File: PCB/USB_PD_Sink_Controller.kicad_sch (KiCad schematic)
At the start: 28 parts, among them J1 USB_C_Receptacle_PowerOnly_6P, J2 JST_01x02_Socket, J3 JST_01x05_Socket, U1 STUSB4500QTR, U2 STL6P3LLH6, U3 STL6P3LLH6

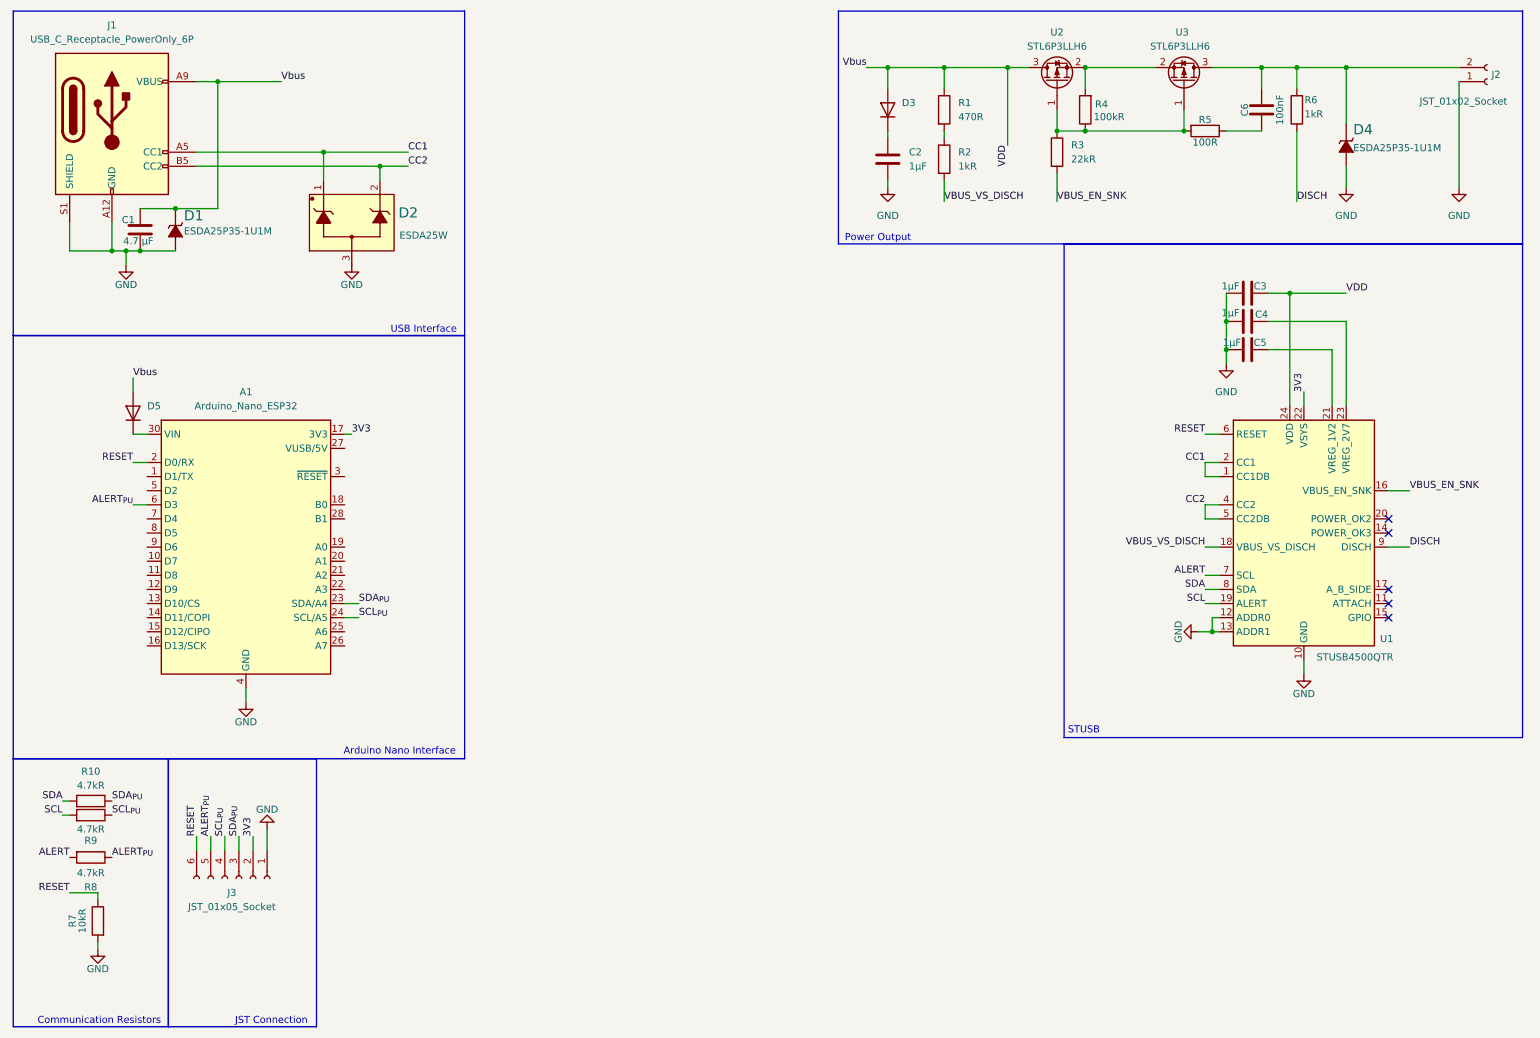
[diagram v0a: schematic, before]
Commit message: Updated PCB
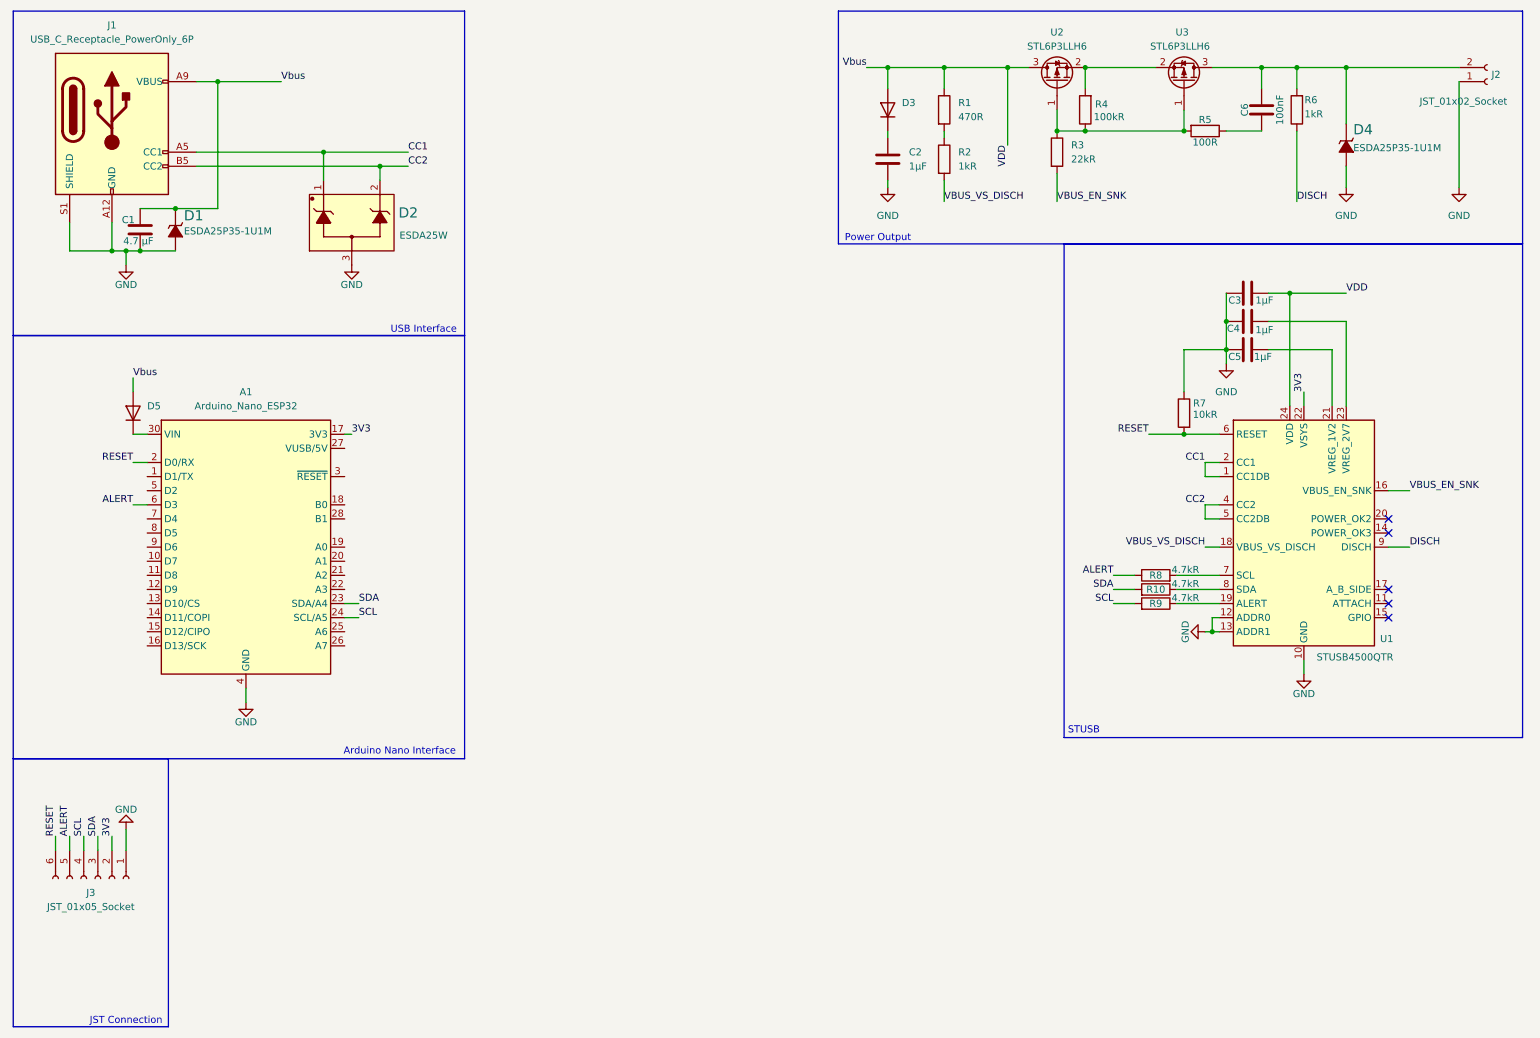
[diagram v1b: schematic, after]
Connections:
- net ALERT_{PU} is gone; now on net ALERT: A1.6 (D3), J3.5 (Pin_5), R8.1
- net ALERT: no longer R8.2, U1.7 (SCL)
- net GND: now also C3.2, C4.2, C5.2, R7.1; no longer C3.1, C4.1, C5.1, R7.2
- net RESET: now also R7.2; no longer R7.1
- net SCL: now also A1.24 (SCL/A5), J3.4 (Pin_4); no longer U1.19 (ALERT)
- net SDA: now also A1.23 (SDA/A4), J3.3 (Pin_3); no longer U1.8 (SDA)
- net VDD: now also C3.1; no longer C3.2
- net at U1.21 (VREG_1V2): now also C5.1; no longer C5.2
- net at U1.23 (VREG_2V7): now also C4.1; no longer C4.2
- removed net SCL_{PU}: A1.24 (SCL/A5), J3.4 (Pin_4), R9.1
- removed net SDA_{PU}: A1.23 (SDA/A4), J3.3 (Pin_3), R10.1
- new net: R8.2, U1.7 (SCL)
- new net: R9.1, U1.19 (ALERT)
- new net: R10.1, U1.8 (SDA)
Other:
- note removed: "Communication Resistors"
- moved on the sheet: C3, C4, C5, J3, R10, R7, R8, R9
